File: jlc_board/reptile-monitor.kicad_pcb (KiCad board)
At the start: 4 copper layers, 38.1 x 84.6 mm, 37 parts, among them J1 1-WIRE, J2 UART, J3 AC_IN, J4 LOAD1, J5 LOAD2, J8 I2C, K1 ALDP105W, K2 ALDP105W, SW1 RST, SW2 BOOT, U1 AP2112M-3.3, U2 NUD3105DMT1G, Y1 32.768KHz 12.5p

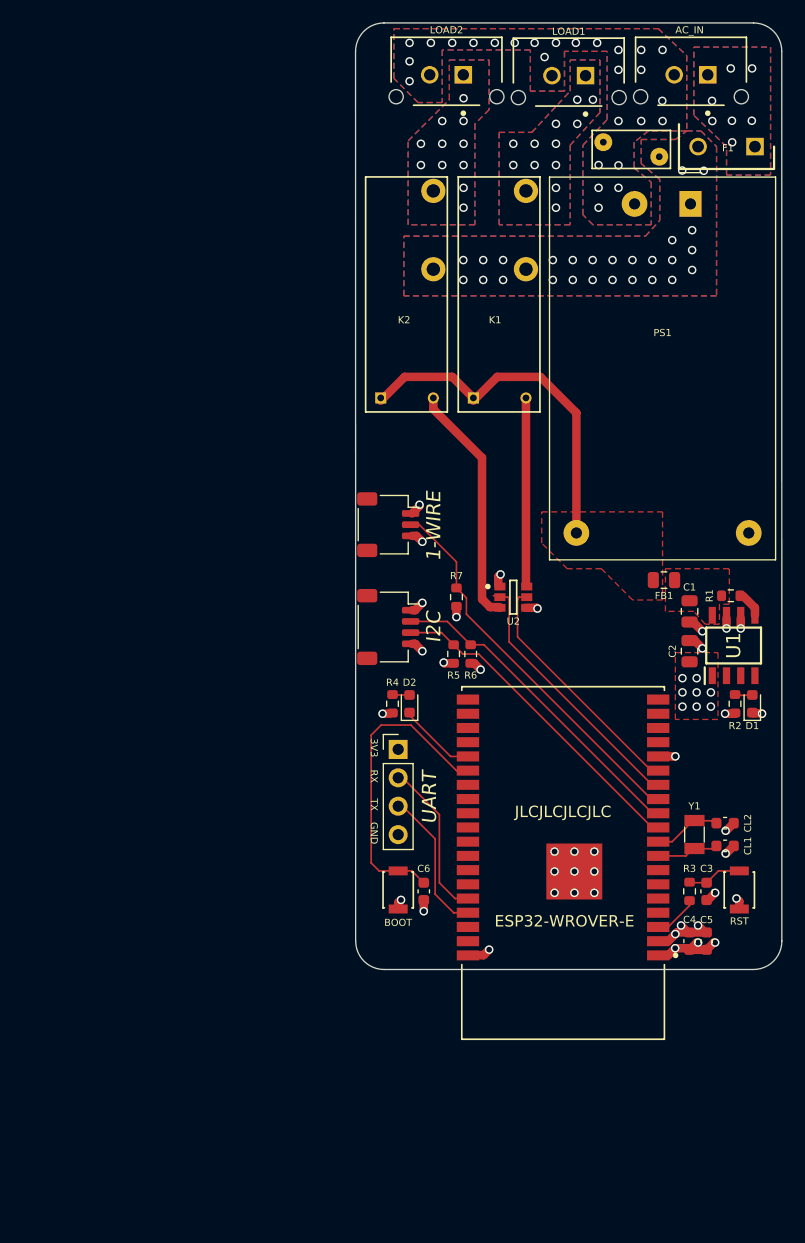
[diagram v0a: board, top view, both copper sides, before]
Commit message: Rev2 - Waffle & Wesley
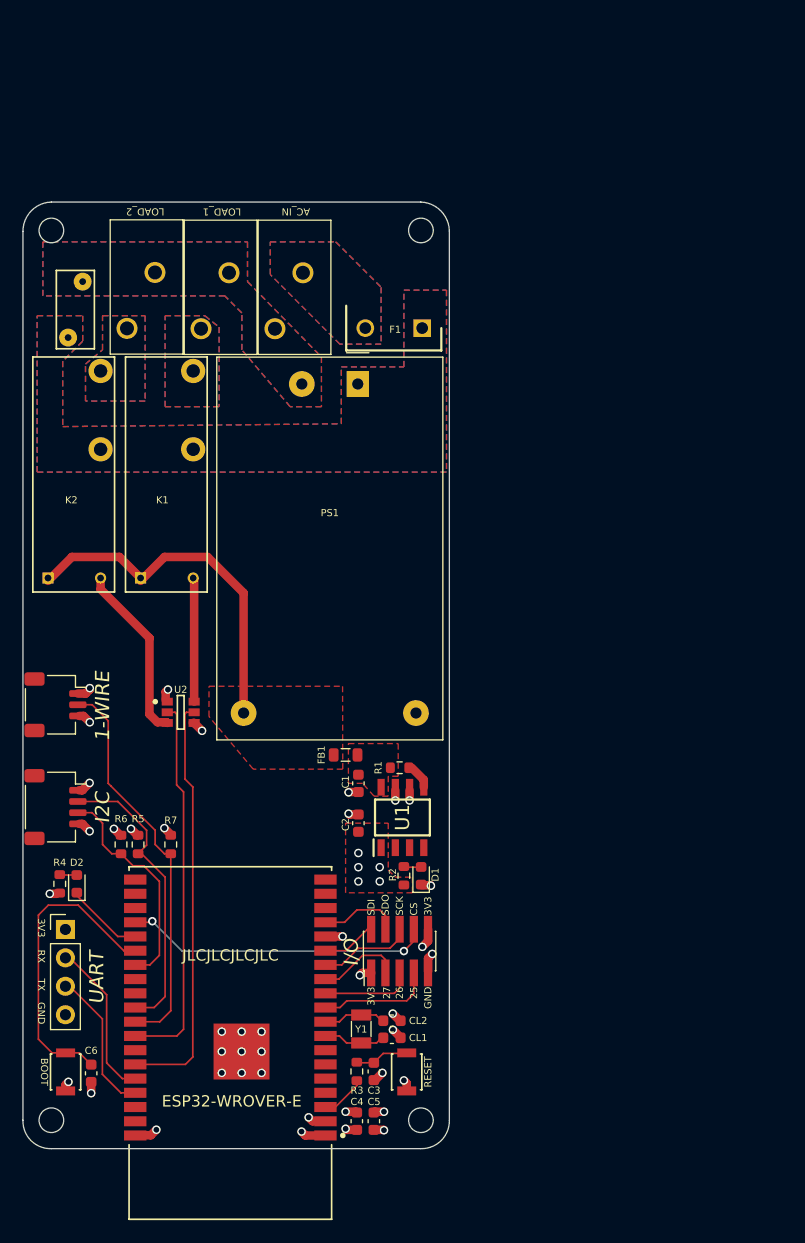
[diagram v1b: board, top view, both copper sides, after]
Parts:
- added J6: I/O, Connector_PinHeader_1.27mm:PinHeader_2x05_P1.27mm_Vertical_SMD, F.Cu at (135.3, 117.7)
- added REF1: MountingHole_2.2mm_M2_ISO7380, MountingHole:MountingHole_2.2mm_M2_ISO7380, F.Cu at (137.2, 53.3)
- added REF1: MountingHole_2.2mm_M2_ISO7380, MountingHole:MountingHole_2.2mm_M2_ISO7380, F.Cu at (104.1, 132.8)
- added REF1: MountingHole_2.2mm_M2_ISO7380, MountingHole:MountingHole_2.2mm_M2_ISO7380, F.Cu at (104.1, 53.3)
- added REF1: MountingHole_2.2mm_M2_ISO7380, MountingHole:MountingHole_2.2mm_M2_ISO7380, F.Cu at (137.2, 132.8)
- C1, C2: footprint Capacitor_SMD:C_0805_2012Metric -> Capacitor_SMD:C_0603_1608Metric
- FB1: footprint Capacitor_SMD:C_0805_2012Metric -> Inductor_SMD:L_0805_2012Metric
- J3: footprint reptile-monitor:Molex-43650-0215-0-0-MFG -> SamacSys_Parts:128340212
- J4: value LOAD1 -> LOAD_1; footprint reptile-monitor:Molex-43650-0215-0-0-MFG -> SamacSys_Parts:128340212
- J5: value LOAD2 -> LOAD_2; footprint reptile-monitor:Molex-43650-0215-0-0-MFG -> SamacSys_Parts:128340212
- SW1: value RST -> RESET
- moved RV1 48.2 mm to (106.9, 57.9), turned to -90 degrees
- moved J3 39.1 mm to (126.6, 57.1), turned to 180 degrees
- moved R6 35.6 mm to (110.4, 108.2), turned to -90 degrees
- moved J4 35.3 mm to (120.0, 57.1), turned to 180 degrees
- moved CL2 34.6 mm to (134.6, 124.0)
- moved Y1 34.5 mm to (131.8, 124.7)
- moved CL1 34.4 mm to (134.6, 125.5)
- moved SW1 33.9 mm to (135.9, 128.5)
- moved C6 33.9 mm to (107.7, 128.7)
- moved SW2 33.9 mm to (105.4, 128.5)
- moved F1 33.9 mm to (137.3, 62.1)
- moved C3 33.8 mm to (133.0, 128.5)
- moved R3 33.8 mm to (131.4, 128.5)
- moved C4 33.8 mm to (131.4, 132.9)
- moved C5 33.8 mm to (133.0, 132.9)
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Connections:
- net /IO0 renamed BOOT
- F1 pad 1: /AC_L -> /FUSED_AC_L
- F1 pad 2: /FUSED_AC_L -> /AC_L
- J1 pad 2: /IO27 -> 1-WIRE
- J4 pad 1: /LOAD1 -> /AC_N
- J4 pad 2: /AC_N -> /LOAD1
- J5 pad 1: /LOAD2 -> /AC_N
- J5 pad 2: /AC_N -> /LOAD2
- J8 pad 2: /IO26 -> SDA
- J8 pad 3: /IO25 -> SCL
- MD1 pad 10: /IO25 -> IO25
- MD1 pad 11: /IO26 -> IO26
- MD1 pad 12: /IO27 -> IO27
- MD1 pad 13: SCLK -> SCK
- MD1 pad 14: MISO -> SDI
- MD1 pad 16: (no net) -> SDO
- MD1 pad 23: (no net) -> CS0
- MD1 pad 26: (no net) -> SCL
- MD1 pad 29: (no net) -> SDA
- MD1 pad 30: (no net) -> 1-WIRE
- MD1 pad 31: (no net) -> L1
- MD1 pad 33: (no net) -> L2
- R5 pad 2: /IO25 -> SDA
- R6 pad 2: /IO26 -> SCL
- R7 pad 2: /IO27 -> 1-WIRE
- U2 pad 2: SCLK -> L1
- U2 pad 5: MISO -> L2
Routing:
- net L2: track 0.00 -> 37.3 mm
- net 1-WIRE: track 0.00 -> 35.5 mm
- net L1: track 0.00 -> 34.0 mm
- net /IO27: track 33.9 -> 0.00 mm
- net /IO25: track 28.7 -> 0.00 mm
- net /IO26: track 28.6 -> 0.00 mm
- net CS0: track 0.00 -> 27.1 mm, vias 0 -> 2
- net SDA: track 0.00 -> 26.9 mm
- net SCLK: track 23.9 -> 0.00 mm
- net MISO: track 21.9 -> 0.00 mm
- net SCL: track 0.00 -> 20.1 mm
- net IO25: track 0.00 -> 10.3 mm
- net IO26: track 0.00 -> 8.58 mm
- net SCK: track 0.00 -> 8.43 mm
- net IO27: track 0.00 -> 7.58 mm
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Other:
- outline, holes or cut-outs redrawn
- board text added: "25"
- board text added: "26"
- board text added: "27"
- board text added: "CS"
- board text added: "SCK"
- board text added: "SDI"
- board text added: "SDO"
